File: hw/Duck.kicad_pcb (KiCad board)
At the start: 2 copper layers, 35.5 x 20.8 mm, 33 parts, among them J1 Conn_01x06, J2 Conn_01x04, J3 USB_C_Receptacle_USB2.0_14P, J4 Conn_01x06, Q1 MMBT3904, Q2 MMBT3904, U1 ESP32-S3-MINI-1, U2 SPX3819M5-L-3-3, U3 INMP441, U4 MAX17048G+T10, U5 CH343P

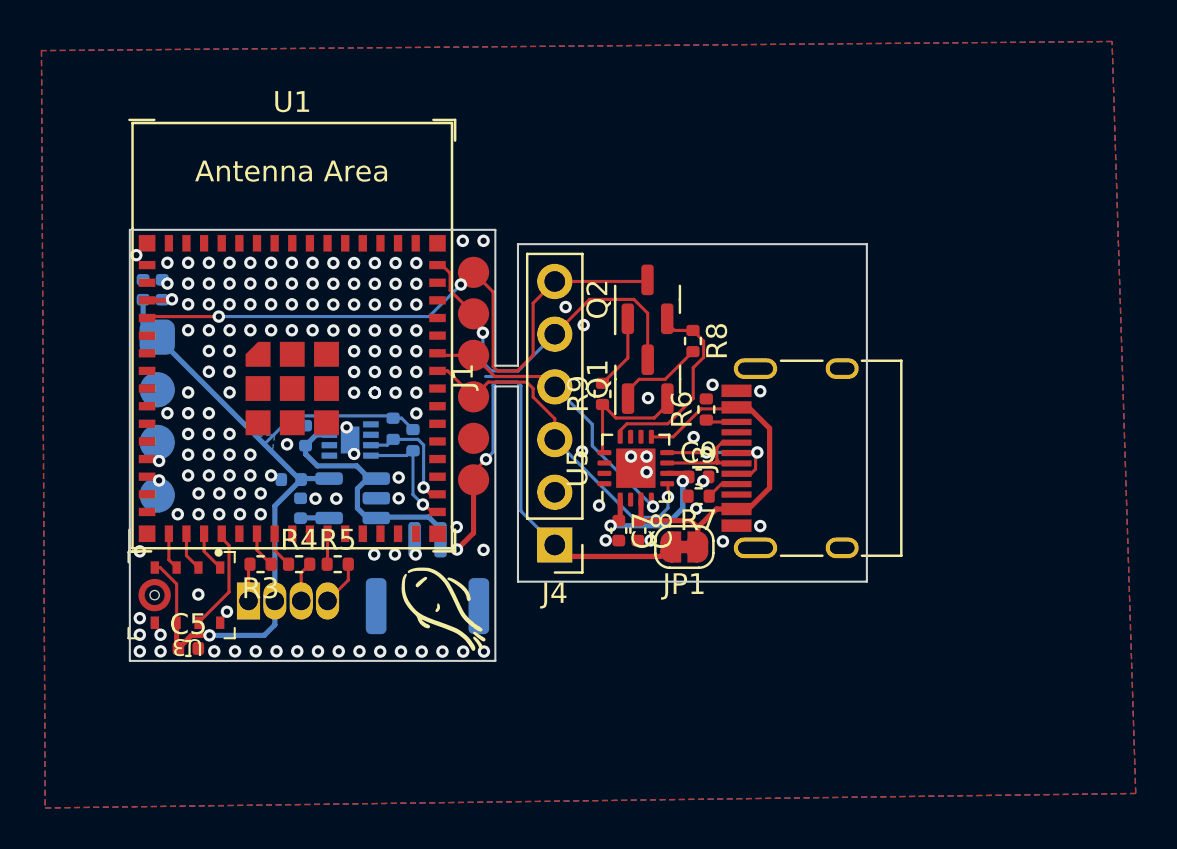
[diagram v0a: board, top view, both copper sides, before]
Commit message: hw: Finalize (...or is it?)
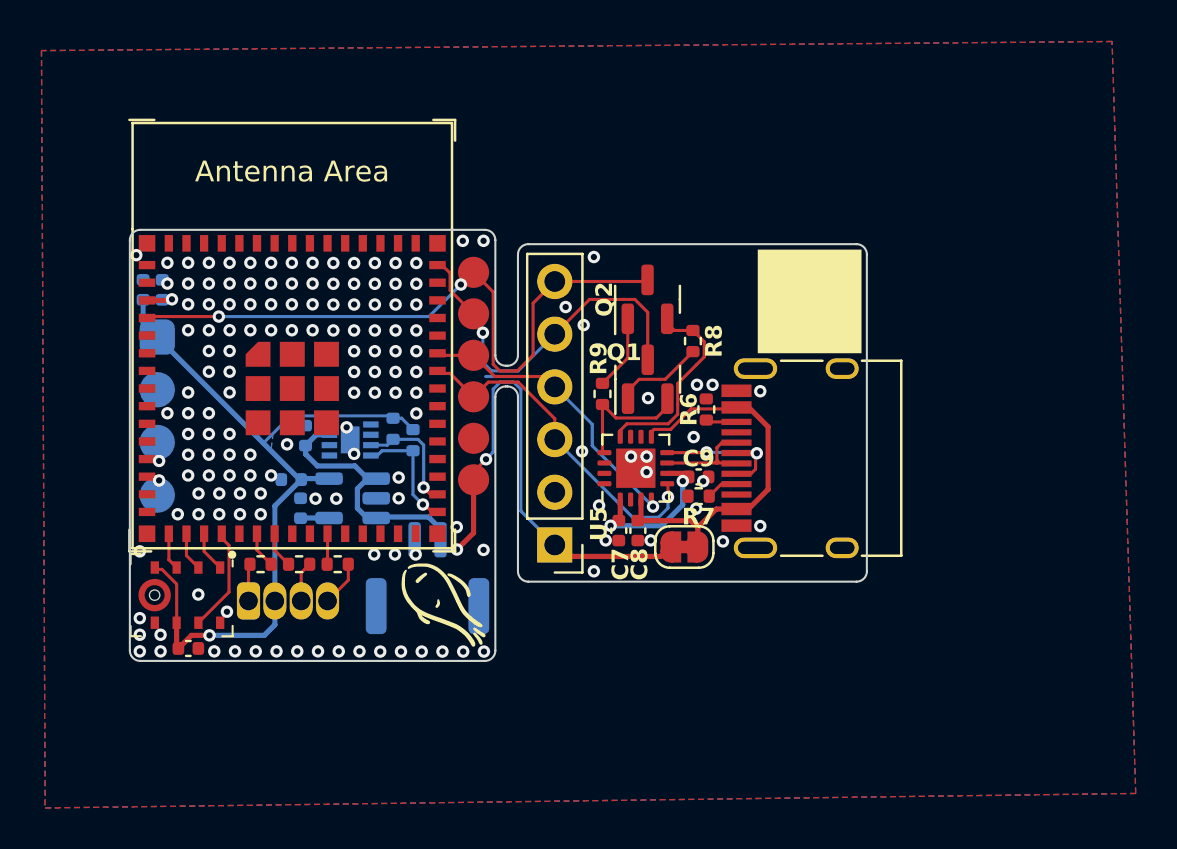
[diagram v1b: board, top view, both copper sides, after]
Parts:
- added G***: LOGO, LOGO, B.Cu at (80.7, 41.6)
- moved G*** 0.20 mm to (71.7, 56.7)
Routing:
- net +BATT: track 37.9 -> 37.3 mm
- net GND: vias 148 -> 150
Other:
- outline, holes or cut-outs redrawn
- board text added: "Round Tracks → Teardrops → Refill & DRC"
